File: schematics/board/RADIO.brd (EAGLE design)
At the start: 30 x 51 mm, 2 parts

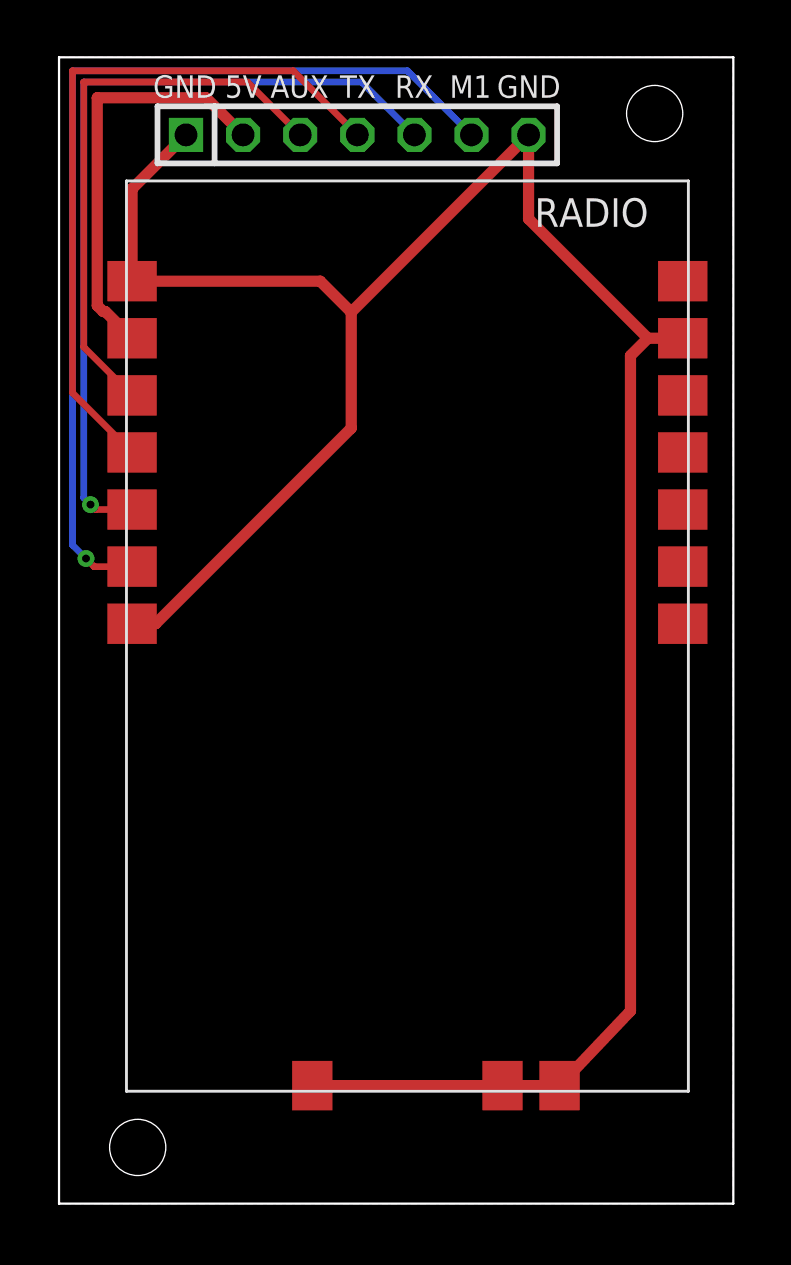
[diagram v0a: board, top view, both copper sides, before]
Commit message: Готова плата RADIO и переделана плата AB
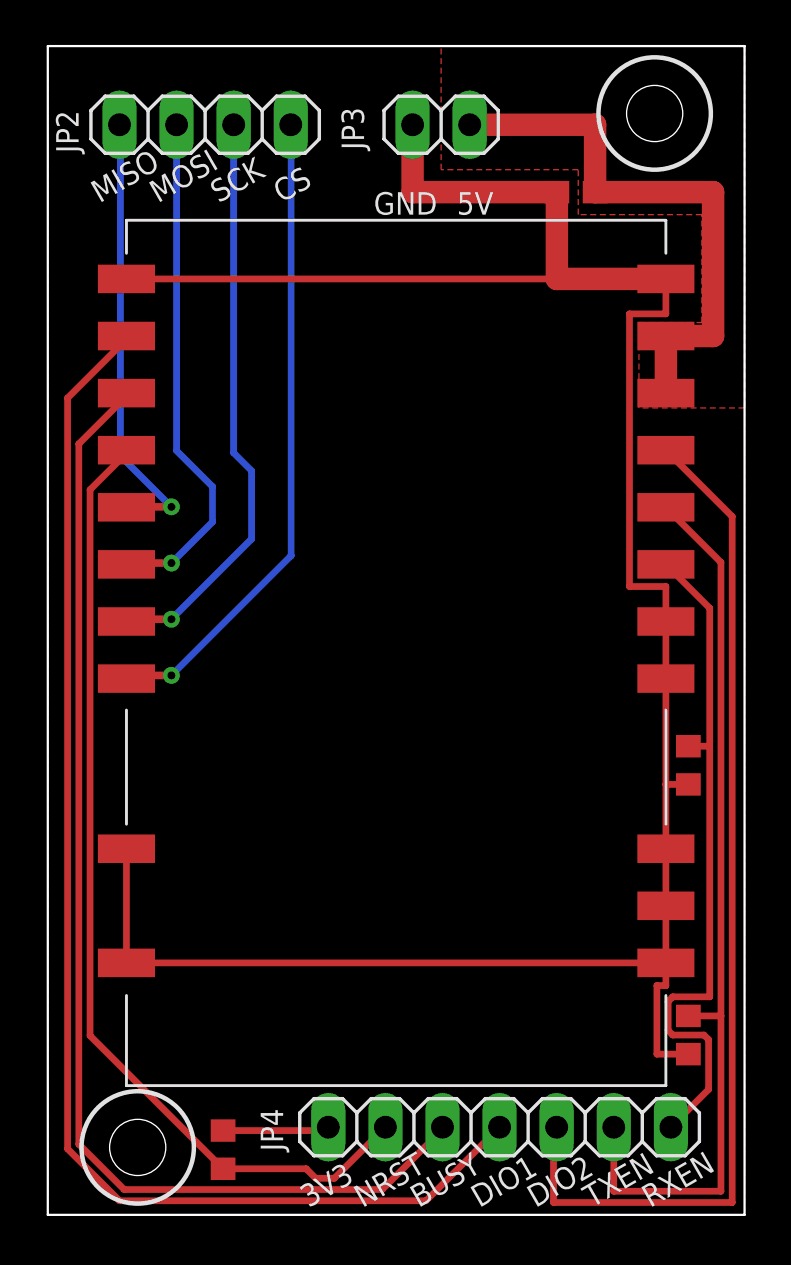
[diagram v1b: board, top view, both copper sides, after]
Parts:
- removed JP1: (no value), pinheadCS:1X07
- removed RADIO: RADIO, CanCubeSat:RADIO
- added C1: 0.1uF, rcl:C0603
- added JP2: (no value), pinhead:1X04
- added JP3: (no value), pinhead:1X02
- added JP4: (no value), pinhead:1X07
- added R1, R2, R3: 5k1, resistor:R0603
- added U$1: E22-400M30S, CanCubeSat:E22-400M30S
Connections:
- removed net AUX: JP1.3, RADIO.P$5
- removed net M1: JP1.6, RADIO.P$2
- removed net RXD: JP1.5, RADIO.P$3
- removed net TXD: JP1.4, RADIO.P$4
- new net 3V3: JP4.1, R1.2
- new net BUSY: JP4.3, U$1.14
- new net CS-RA: JP2.1, U$1.19
- new net DIO1: JP4.4, U$1.13
- new net DIO2: JP4.5, U$1.8
- new net MISO: JP2.4, U$1.16
- new net MOSI: JP2.3, U$1.17
- new net NRST: JP4.2, R1.1, U$1.15
- new net RX-EN: JP4.7, R2.1, U$1.6
- new net SCK: JP2.2, U$1.18
- new net TX-EN: JP4.6, R3.1, U$1.7
- net 5V: now also C1.1, JP3.1, U$1.10, U$1.9; no longer JP1.2, RADIO.P$6
- net GND: now also C1.2, JP3.2, R2.2, R3.2, U$1.1, U$1.11, U$1.12, U$1.2, U$1.20, U$1.22, U$1.3, U$1.4, U$1.5; no longer JP1.1, JP1.7, RADIO.P$1, RADIO.P$15, RADIO.P$16, RADIO.P$17, RADIO.P$7, RADIO.P$9
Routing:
- net DIO1: track 0.00 -> 58.8 mm
- net BUSY: track 0.00 -> 52.5 mm
- net DIO2: track 0.00 -> 46.0 mm
- net NRST: track 0.00 -> 43.4 mm
- net M1: track 43.1 -> 0.00 mm, vias 1 -> 0
- net TX-EN: track 0.00 -> 40.5 mm
- net RXD: track 36.5 -> 0.00 mm, vias 1 -> 0
- net TXD: track 31.9 -> 0.00 mm
- net RX-EN: track 0.00 -> 30.8 mm
- net CS-RA: track 0.00 -> 28.8 mm, vias 0 -> 1
- net SCK: track 0.00 -> 25.9 mm, vias 0 -> 1
- net AUX: track 25.4 -> 0.00 mm
- net MOSI: track 0.00 -> 22.9 mm, vias 0 -> 1
- net MISO: track 0.00 -> 20.0 mm, vias 0 -> 1
- net 5V: track 18.6 -> 24.9 mm
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- added copper zone on layer 1, net 5V
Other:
- board size 30 x 51 mm -> 31 x 52 mm
- board text added: "3V3"
- board text added: "BUSY"
- board text added: "CS"
- board text added: "DIO1"
- board text added: "DIO2"
- board text added: "MISO"
- board text added: "MOSI"
- board text added: "NRST"
- board text added: "RXEN"
- board text added: "SCK"
- board text added: "TXEN"
- board text removed: "AUX"
- board text removed: "M1"
- board text removed: "RX"
- board text removed: "TX"
